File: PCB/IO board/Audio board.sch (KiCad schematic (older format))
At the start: 6 parts, among them J101 Screen_Standoff, J102 Screen_Standoff, J103 Standoff_MaGee, J104 Screen_Standoff, J105 Screen_Standoff, X101 Cap'n_MaGee

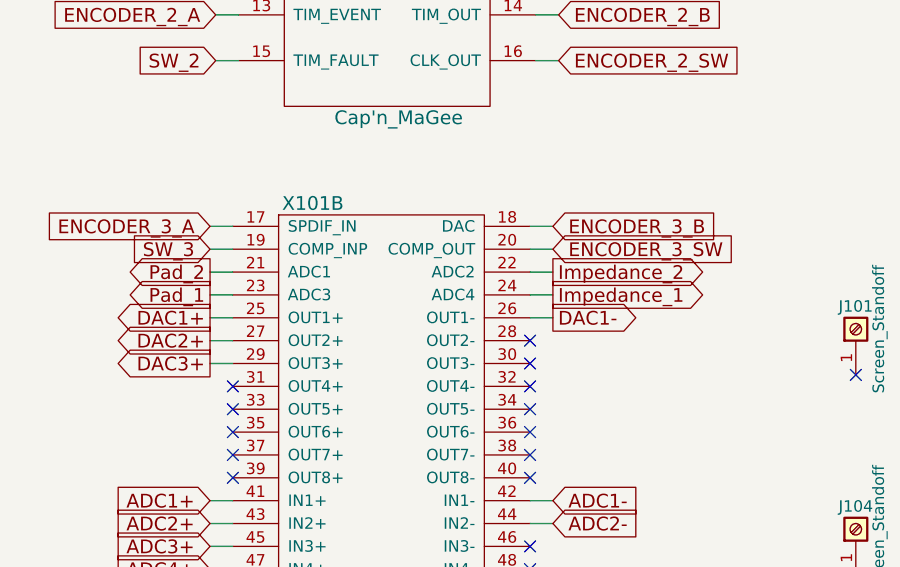
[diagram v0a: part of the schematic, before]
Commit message: IO board Rev 1.0 RC-1
Board for inspection by Supervisor
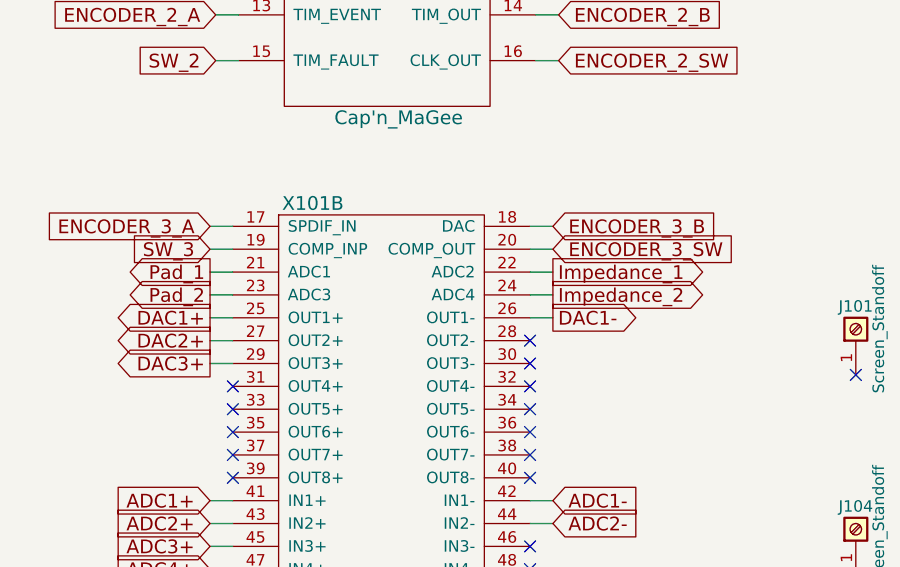
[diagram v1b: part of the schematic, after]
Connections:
- net Impedance_1: now also X101.22 (ADC2); no longer X101.24 (ADC4)
- net Impedance_2: now also X101.24 (ADC4); no longer X101.22 (ADC2)
- net Pad_1: now also X101.21 (ADC1); no longer X101.23 (ADC3)
- net Pad_2: now also X101.23 (ADC3); no longer X101.21 (ADC1)
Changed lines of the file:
@@
 	1    0    0    -1
 $EndComp
+Text GLabel 1325 5425 0    60   Output ~ 0
+Pad_1
+Text GLabel 2825 5425 2    60   Output ~ 0
+Impedance_1
+Text GLabel 2825 5525 2    60   Output ~ 0
+Impedance_2
 Text GLabel 1325 5525 0    60   Output ~ 0
-Pad_1
-Text GLabel 2825 5525 2    60   Output ~ 0
-Impedance_1
-Text GLabel 2825 5425 2    60   Output ~ 0
-Impedance_2
-Text GLabel 1325 5425 0    60   Output ~ 0
 Pad_2
 Text GLabel 1350 3700 0    60   Output ~ 0
